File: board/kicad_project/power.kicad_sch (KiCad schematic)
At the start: 6 parts, among them IC2 ME6211C33M5G-N, U2 AMS1117-3.3

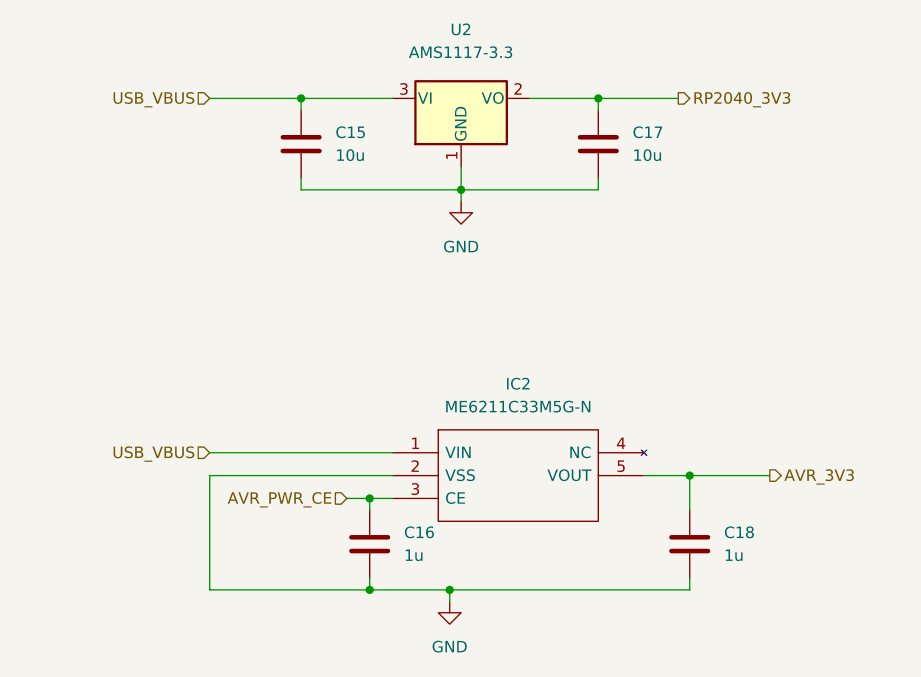
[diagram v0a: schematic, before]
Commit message: Initial board design
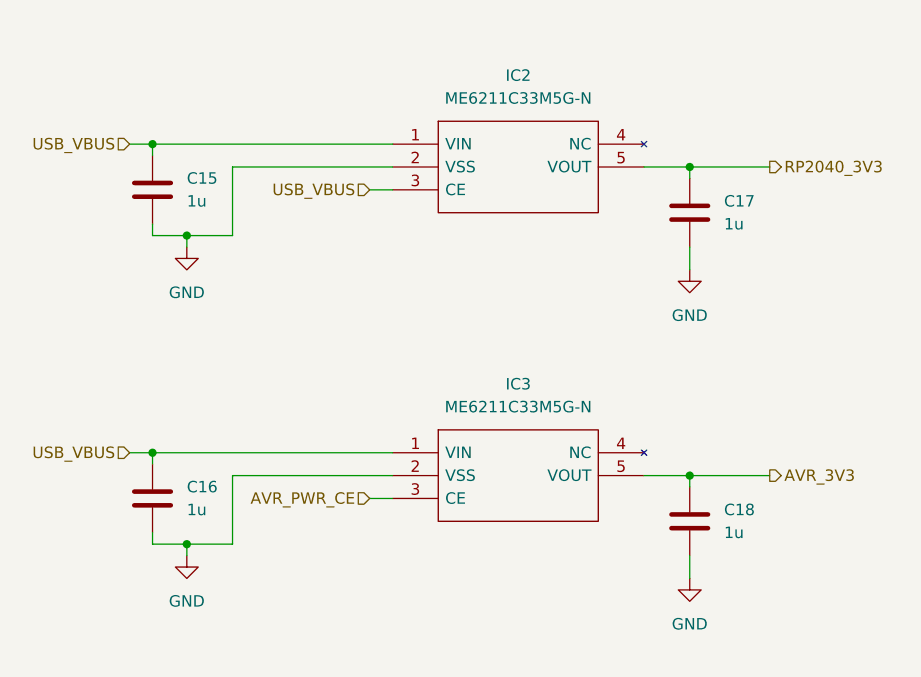
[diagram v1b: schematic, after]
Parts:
- removed U2: AMS1117-3.3, Package_TO_SOT_SMD:SOT-223-3_TabPin2, symbol Regulator_Linear:AMS1117-3.3
- added IC2: ME6211C33M5G-N, Package_TO_SOT_SMD:SOT-23-5, symbol ME6211C33M5G-N:ME6211C33M5G-N
- C15, C17: value 10u -> 1u
- C16, C18: footprint Capacitor_SMD:C_0603_1608Metric -> Capacitor_SMD:C_0805_2012Metric
- renumbered IC2 to IC3
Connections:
- net AVR_PWR_CE: no longer C16.1
- net GND: now also IC2.2 (VSS)
- net RP2040_3V3: now also IC2.5 (VOUT)
- net USB_VBUS: now also C16.1, IC2.1 (VIN), IC2.3 (CE)
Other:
- moved on the sheet: C18

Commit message: Added lcsc part numbers
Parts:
- C15, C16, C17, C18: LCSC Part (none) -> C28323
- IC2, IC3: LCSC Part (none) -> C82942
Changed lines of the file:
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@@
+      (effects (font (size 1.27 1.27)) hide)
+    )
+    (property "LCSC Part" "C28323" (id 4) (at 102.87 60.96 0)
       (effects (font (size 1.27 1.27)) hide)
     )
@@
       (effects (font (size 1.27 1.27)) hide)
     )
+    (property "LCSC Part" "C28323" (id 4) (at 102.87 95.25 0)
+      (effects (font (size 1.27 1.27)) hide)
+    )
     (pin "1")
     (pin "2")
@@
       (effects (font (size 1.27 1.27)) hide)
     )
+    (property "LCSC Part" "C28323" (id 4) (at 162.56 63.5 0)
+      (effects (font (size 1.27 1.27)) hide)
+    )
     (pin "1")
     (pin "2")
@@
     )
     (property "Datasheet" "~" (id 3) (at 162.56 97.79 0)
+      (effects (font (size 1.27 1.27)) hide)
+    )
+    (property "LCSC Part" "C28323" (id 4) (at 162.56 97.79 0)
       (effects (font (size 1.27 1.27)) hide)
     )
@@
     (property "Arrow Price/Stock" "" (id 11) (at 153.67 76.2 0)
       (effects (font (size 1.27 1.27)) (justify left) hide)
+    )
+    (property "LCSC Part" "C82942" (id 12) (at 129.54 55.88 0)
+      (effects (font (size 1.27 1.27)) hide)
     )
     (pin "1")
@@
       (effects (font (size 1.27 1.27)) (justify left) hide)
     )
+    (property "LCSC Part" "C82942" (id 12) (at 129.54 90.17 0)
+      (effects (font (size 1.27 1.27)) hide)
+    )
     (pin "1")
